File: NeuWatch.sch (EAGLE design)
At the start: 61 parts, among them IC1 SAMD21G18A-AUT, IC3 TPS2115, IC4 SIP32401A, IC5 MC74VHC1G14DFT, Y1 32,768Khz

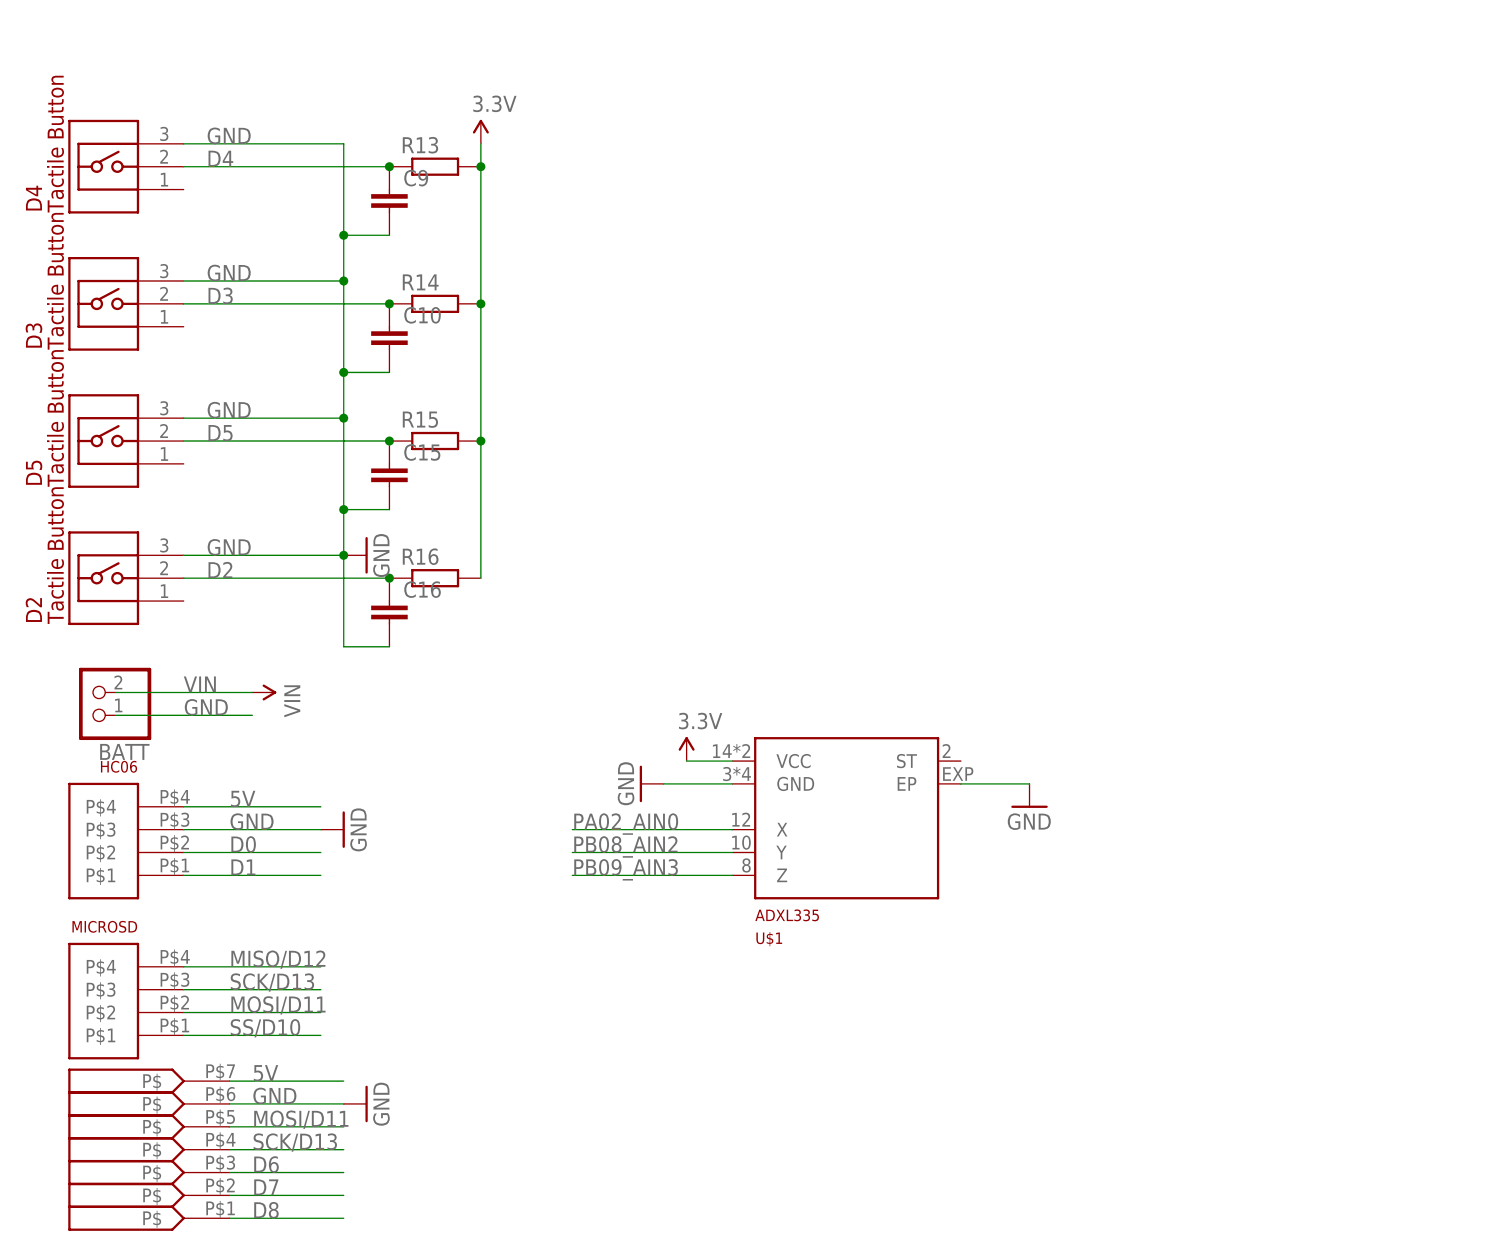
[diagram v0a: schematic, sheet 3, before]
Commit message: added batsense
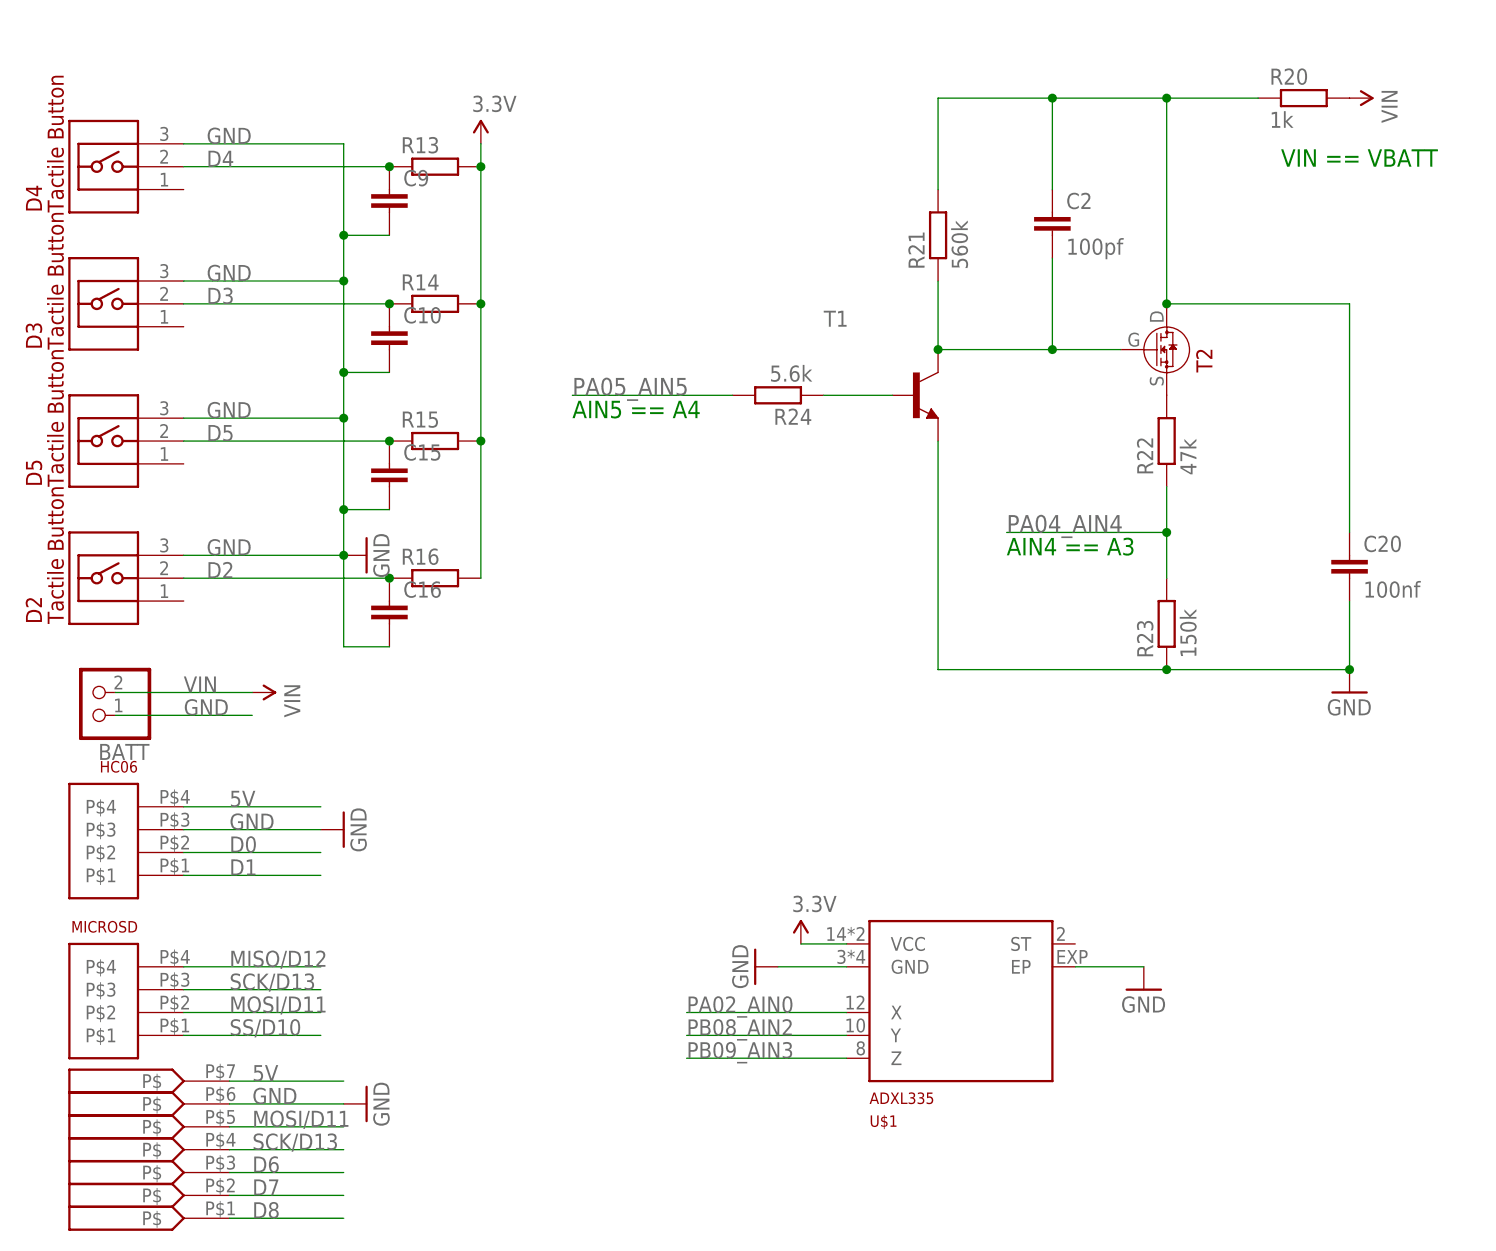
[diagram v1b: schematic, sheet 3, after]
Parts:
- added C2: 100pf, AtomTech:CAPACITORC0402
- added C20: 100nf, AtomTech:CAPACITORC0402
- added R20: 1k, rcl:R-EU_R0402
- added R21: 560k, rcl:R-EU_R0402
- added R22: 47k, rcl:R-EU_R0402
- added R23: 150k, rcl:R-EU_R0402
- added R24: 5.6k, rcl:R-EU_R0402
- added T1: (no value), transistor:BC846BLT1-NPN-SOT23-BEC
- added T2: 2N7002_ALT, AtomTech:2N7002_ALT
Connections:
- new net N$14: R22.2, T2.S
- new net N$5: C2.2, R21.1, T1.C, T2.G
- new net N$8: R24.1, T1.B
- new net N$9: C2.1, C20.1, R20.1, R21.2, T2.D
- net GND: now also C20.2, R23.1, T1.E
- net PA04_AIN4: now also R22.1, R23.2
- net PA05_AIN5: now also R24.2
- net VIN: now also R20.2
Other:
- note added: "AIN4 == A3"
- note added: "AIN5 == A4"
- note added: "VIN == VBATT"
- moved on the sheet: U$1
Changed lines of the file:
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@@
 <part name="SUPPLY17" library="SparkFun-Aesthetics" deviceset="3.3V" device=""/>
 <part name="C19" library="AtomTech" deviceset="CAPACITOR" device="C0402" value="100nf"/>
+<part name="R20" library="rcl" deviceset="R-EU_" device="R0402" value="1k"/>
+<part name="R21" library="rcl" deviceset="R-EU_" device="R0402" value="560k"/>
+<part name="C2" library="AtomTech" deviceset="CAPACITOR" device="C0402" value="100pf"/>
+<part name="C20" library="AtomTech" deviceset="CAPACITOR" device="C0402" value="100nf"/>
+<part name="R22" library="rcl" deviceset="R-EU_" device="R0402" value="47k"/>
+<part name="R23" library="rcl" deviceset="R-EU_" device="R0402" value="150k"/>
+<part name="T1" library="transistor" deviceset="*-NPN-" device="SOT23-BEC" technology="BC846BLT1"/>
+<part name="R24" library="rcl" deviceset="R-EU_" device="R0402" value="5.6k"/>
+<part name="T2" library="AtomTech" deviceset="2N7002_ALT" device=""/>
+<part name="SUPPLY3" library="SparkFun-Aesthetics" deviceset="VIN" device=""/>
+<part name="GND1" library="supply1" deviceset="GND" device=""/>
 </parts>
 <sheets>
@@
 <sheet>
 <plain>
+<text x="73.66" y="129.54" size="1.9304" layer="91">AIN5 == A4</text>
+<text x="121.92" y="114.3" size="1.9304" layer="91">AIN4 == A3</text>
+<text x="152.4" y="157.48" size="1.9304" layer="91">VIN == VBATT</text>
 </plain>
 <instances>
@@
 <instance part="C15" gate="G$1" x="53.34" y="124.46"/>
 <instance part="C16" gate="G$1" x="53.34" y="109.22"/>
-<instance part="U$1" gate="G$1" x="104.14" y="83.82"/>
-<instance part="SUPPLY5" gate="G$1" x="86.36" y="91.44"/>
-<instance part="GND26" gate="1" x="81.28" y="88.9" rot="R270"/>
-<instance part="GND27" gate="1" x="124.46" y="86.36"/>
+<instance part="U$1" gate="G$1" x="116.84" y="63.5"/>
+<instance part="SUPPLY5" gate="G$1" x="99.06" y="71.12"/>
+<instance part="GND26" gate="1" x="93.98" y="68.58" rot="R270"/>
+<instance part="GND27" gate="1" x="137.16" y="66.04"/>
+<instance part="R20" gate="G$1" x="154.94" y="165.1"/>
+<instance part="R21" gate="G$1" x="114.3" y="149.86" rot="R90"/>
+<instance part="C2" gate="G$1" x="127" y="152.4"/>
+<instance part="C20" gate="G$1" x="160.02" y="114.3"/>
+<instance part="R22" gate="G$1" x="139.7" y="127" rot="R90"/>
+<instance part="R23" gate="G$1" x="139.7" y="106.68" rot="R90"/>
+<instance part="T1" gate="G$1" x="111.76" y="132.08"/>
+<instance part="R24" gate="G$1" x="96.52" y="132.08" rot="R180"/>
+<instance part="T2" gate="G$1" x="139.7" y="137.16"/>
+<instance part="SUPPLY3" gate="G$1" x="160.02" y="165.1" rot="R270"/>
+<instance part="GND1" gate="1" x="160.02" y="99.06"/>
 </instances>
 <busses>
@@
 <pinref part="U$1" gate="G$1" pin="GND"/>
 <pinref part="GND26" gate="1" pin="GND"/>
-<wire x1="83.82" y1="88.9" x2="91.44" y2="88.9" width="0.1524" layer="91"/>
+<wire x1="96.52" y1="68.58" x2="104.14" y2="68.58" width="0.1524" layer="91"/>
 </segment>
 <segment>
 <pinref part="U$1" gate="G$1" pin="EP"/>
 <pinref part="GND27" gate="1" pin="GND"/>
-<wire x1="124.46" y1="88.9" x2="116.84" y2="88.9" width="0.1524" layer="91"/>
+<wire x1="137.16" y1="68.58" x2="129.54" y2="68.58" width="0.1524" layer="91"/>
+</segment>
+<segment>
+<pinref part="C20" gate="G$1" pin="2"/>
+<wire x1="160.02" y1="109.22" x2="160.02" y2="101.6" width="0.1524" layer="91"/>
+<pinref part="R23" gate="G$1" pin="1"/>
+<wire x1="160.02" y1="101.6" x2="139.7" y2="101.6" width="0.1524" layer="91"/>
+<pinref part="T1" gate="G$1" pin="E"/>
+<wire x1="139.7" y1="101.6" x2="114.3" y2="101.6" width="0.1524" layer="91"/>
+<wire x1="114.3" y1="101.6" x2="114.3" y2="127" width="0.1524" layer="91"/>
+<junction x="139.7" y="101.6"/>
+<pinref part="GND1" gate="1" pin="GND"/>
+<junction x="160.02" y="101.6"/>
 </segment>
 </net>
@@
 <label x="30.48" y="99.06" size="1.778" layer="95"/>
 <pinref part="SUPPLY16" gate="G$1" pin="VIN"/>
+</segment>
+<segment>
+<pinref part="R20" gate="G$1" pin="2"/>
+<pinref part="SUPPLY3" gate="G$1" pin="VIN"/>
 </segment>
 </net>
@@
 <pinref part="U$1" gate="G$1" pin="VCC"/>
 <pinref part="SUPPLY5" gate="G$1" pin="3.3V"/>
-<wire x1="86.36" y1="91.44" x2="91.44" y2="91.44" width="0.1524" layer="91"/>
+<wire x1="99.06" y1="71.12" x2="104.14" y2="71.12" width="0.1524" layer="91"/>
 </segment>
 </net>
@@
 <segment>
 <pinref part="U$1" gate="G$1" pin="X"/>
-<wire x1="73.66" y1="83.82" x2="91.44" y2="83.82" width="0.1524" layer="91"/>
-<label x="73.66" y="83.82" size="1.778" layer="95"/>
+<wire x1="86.36" y1="63.5" x2="104.14" y2="63.5" width="0.1524" layer="91"/>
+<label x="86.36" y="63.5" size="1.778" layer="95"/>
 </segment>
 </net>
@@
 <segment>
 <pinref part="U$1" gate="G$1" pin="Y"/>
-<wire x1="73.66" y1="81.28" x2="91.44" y2="81.28" width="0.1524" layer="91"/>
-<label x="73.66" y="81.28" size="1.778" layer="95"/>
+<wire x1="86.36" y1="60.96" x2="104.14" y2="60.96" width="0.1524" layer="91"/>
+<label x="86.36" y="60.96" size="1.778" layer="95"/>
 </segment>
 </net>
@@
 <segment>
 <pinref part="U$1" gate="G$1" pin="Z"/>
-<wire x1="73.66" y1="78.74" x2="91.44" y2="78.74" width="0.1524" layer="91"/>
-<label x="73.66" y="78.74" size="1.778" layer="95"/>
-</segment>
-</net>
+<wire x1="86.36" y1="58.42" x2="104.14" y2="58.42" width="0.1524" layer="91"/>
+<label x="86.36" y="58.42" size="1.778" layer="95"/>
+</segment>
+</net>
+<net name="N$5" class="0">
+<segment>
+<pinref part="R21" gate="G$1" pin="1"/>
+<pinref part="T1" gate="G$1" pin="C"/>
+<wire x1="114.3" y1="144.78" x2="114.3" y2="137.16" width="0.1524" layer="91"/>
+<pinref part="C2" gate="G$1" pin="2"/>
+<wire x1="127" y1="147.32" x2="127" y2="137.16" width="0.1524" layer="91"/>
+<wire x1="127" y1="137.16" x2="114.3" y2="137.16" width="0.1524" layer="91"/>
+<junction x="114.3" y="137.16"/>
+<pinref part="T2" gate="G$1" pin="G"/>
+<wire x1="127" y1="137.16" x2="134.62" y2="137.16" width="0.1524" layer="91"/>
+<junction x="127" y="137.16"/>
+</segment>
+</net>
+<net name="N$8" class="0">
+<segment>
+<pinref part="T1" gate="G$1" pin="B"/>
+<pinref part="R24" gate="G$1" pin="1"/>
+<wire x1="101.6" y1="132.08" x2="109.22" y2="132.08" width="0.1524" layer="91"/>
+</segment>
+</net>
+<net name="N$9" class="0">
+<segment>
+<pinref part="R20" gate="G$1" pin="1"/>
+<pinref part="R21" gate="G$1" pin="2"/>
+<wire x1="149.86" y1="165.1" x2="139.7" y2="165.1" width="0.1524" layer="91"/>
+<wire x1="139.7" y1="165.1" x2="127" y2="165.1" width="0.1524" layer="91"/>
+<wire x1="127" y1="165.1" x2="114.3" y2="165.1" width="0.1524" layer="91"/>
+<wire x1="114.3" y1="165.1" x2="114.3" y2="154.94" width="0.1524" layer="91"/>
+<pinref part="C2" gate="G$1" pin="1"/>
+<wire x1="127" y1="154.94" x2="127" y2="165.1" width="0.1524" layer="91"/>
+<junction x="127" y="165.1"/>
+<wire x1="139.7" y1="165.1" x2="139.7" y2="142.24" width="0.1524" layer="91"/>
+<junction x="139.7" y="165.1"/>
+<pinref part="C20" gate="G$1" pin="1"/>
+<wire x1="139.7" y1="142.24" x2="160.02" y2="142.24" width="0.1524" layer="91"/>
+<wire x1="160.02" y1="142.24" x2="160.02" y2="116.84" width="0.1524" layer="91"/>
+<pinref part="T2" gate="G$1" pin="D"/>
+<junction x="139.7" y="142.24"/>
+</segment>
+</net>
+<net name="N$14" class="0">
+<segment>
+<pinref part="T2" gate="G$1" pin="S"/>
+<pinref part="R22" gate="G$1" pin="2"/>
+</segment>
+</net>
+<net name="PA04_AIN4" class="0">
+<segment>
+<pinref part="R23" gate="G$1" pin="2"/>
+<pinref part="R22" gate="G$1" pin="1"/>
+<wire x1="139.7" y1="111.76" x2="139.7" y2="116.84" width="0.1524" layer="91"/>
+<wire x1="139.7" y1="116.84" x2="139.7" y2="121.92" width="0.1524" layer="91"/>
+<wire x1="139.7" y1="116.84" x2="121.92" y2="116.84" width="0.1524" layer="91"/>
+<junction x="139.7" y="116.84"/>
+<label x="121.92" y="116.84" size="1.9304" layer="95"/>
+</segment>
+</net>
+<net name="PA05_AIN5" class="0">
+<segment>
+<pinref part="R24" gate="G$1" pin="2"/>
+<wire x1="73.66" y1="132.08" x2="91.44" y2="132.08" width="0.1524" layer="91"/>
+<label x="73.66" y="132.08" size="1.9304" layer="95"/>
+</segment>
+</net>
